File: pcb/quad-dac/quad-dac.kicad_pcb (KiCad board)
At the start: 2 copper layers, 90 x 90 mm, 18 parts, among them J1 Power+SPI, J2 CV_OUT, U1 AD5754R

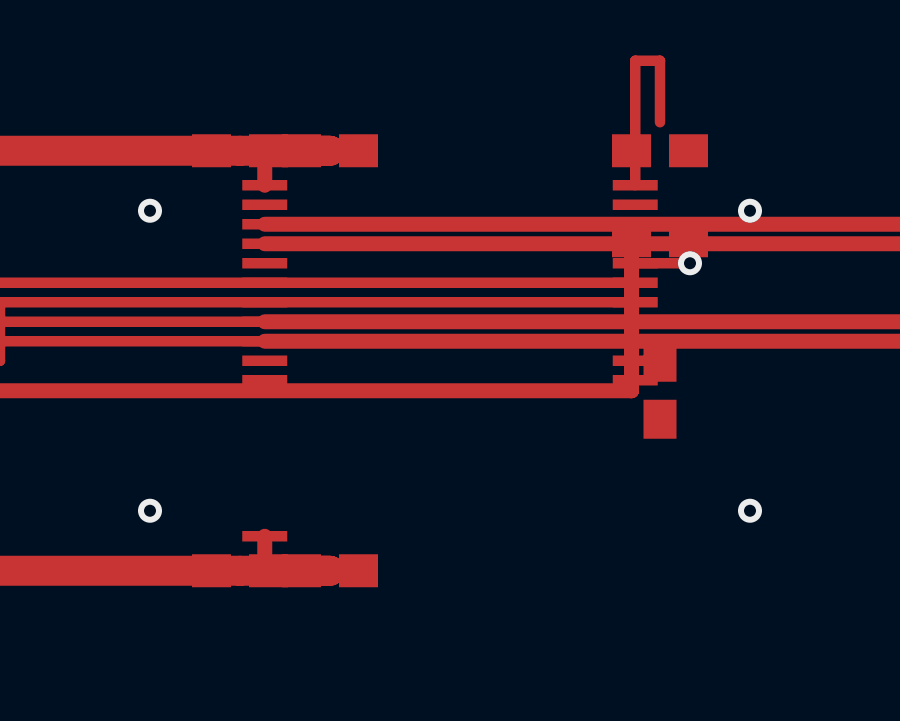
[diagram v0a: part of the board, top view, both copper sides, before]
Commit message: pcbs
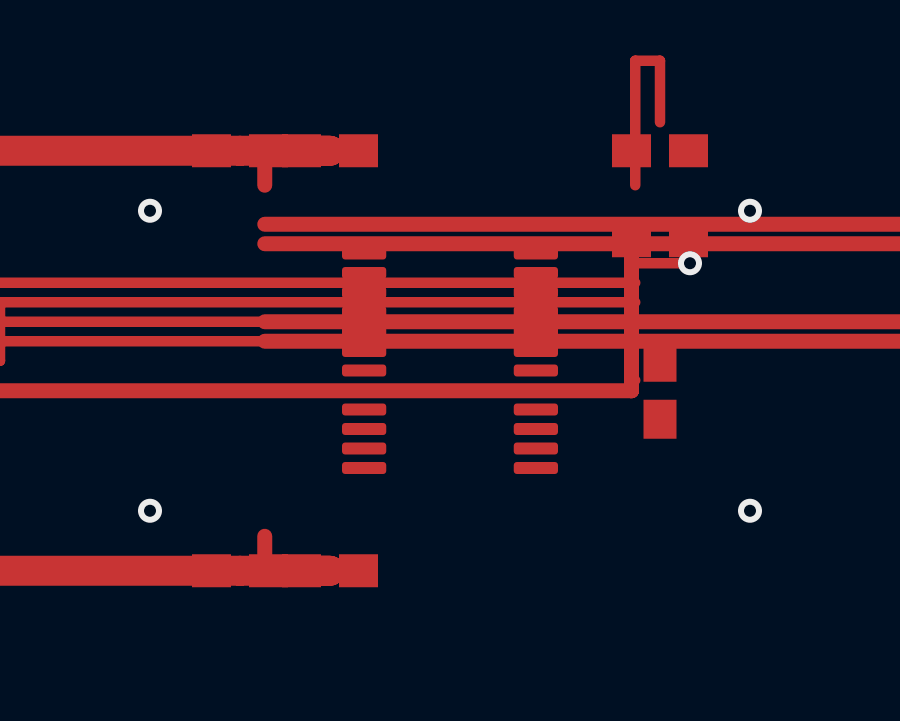
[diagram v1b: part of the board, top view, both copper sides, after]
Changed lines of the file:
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@@
   ;; =========================================================================
   ;; ── U1: AD5754R — TSSOP-24 ────────────────────────────────────────────
+  ;; Pin mapping: AD5754R pin 1 (AVSS) at top-left → KiCad pad 1 at (-2.8625, 3.575)
+  ;; Counter-clockwise: pads 1-12 left side (top→bottom), pads 13-24 right side (bottom→top)
   (footprint "Package_SO:TSSOP-24_4.4x7.8mm_P0.65mm"
     (layer "F.Cu")
@@
     (property "Value" "AD5754R" (at 45 52 0) (layer "F.Fab")
       (effects (font (size 1.0 1.0) (thickness 0.15))))
-    (pad "1" smd rect (at -6.175 -5.85 0) (size 1.5 0.35) (layers "F.Cu" "F.Paste" "F.Mask") (net 2))
-    (pad "2" smd rect (at -6.175 -5.2 0) (size 1.5 0.35) (layers "F.Cu" "F.Paste" "F.Mask") (net 4))
-    (pad "3" smd rect (at -6.175 -4.55 0) (size 1.5 0.35) (layers "F.Cu" "F.Paste" "F.Mask") (net 9))
-    (pad "4" smd rect (at -6.175 -3.9 0) (size 1.5 0.35) (layers "F.Cu" "F.Paste" "F.Mask") (net 10))
-    (pad "5" smd rect (at -6.175 -3.25 0) (size 1.5 0.35) (layers "F.Cu" "F.Paste" "F.Mask") (net 0))
-    (pad "6" smd rect (at -6.175 -2.6 0) (size 1.5 0.35) (layers "F.Cu" "F.Paste" "F.Mask") (net 0))
-    (pad "7" smd rect (at -6.175 -1.95 0) (size 1.5 0.35) (layers "F.Cu" "F.Paste" "F.Mask") (net 0))
-    (pad "8" smd rect (at -6.175 -1.3 0) (size 1.5 0.35) (layers "F.Cu" "F.Paste" "F.Mask") (net 11))
-    (pad "9" smd rect (at -6.175 -0.65 0) (size 1.5 0.35) (layers "F.Cu" "F.Paste" "F.Mask") (net 12))
-    (pad "10" smd rect (at -6.175 0.0 0) (size 1.5 0.35) (layers "F.Cu" "F.Paste" "F.Mask") (net 4))
-    (pad "11" smd rect (at -6.175 0.65 0) (size 1.5 0.35) (layers "F.Cu" "F.Paste" "F.Mask") (net 4))
-    (pad "12" smd rect (at 6.175 0.65 0) (size 1.5 0.35) (layers "F.Cu" "F.Paste" "F.Mask") (net 3))
-    (pad "13" smd rect (at 6.175 0.0 0) (size 1.5 0.35) (layers "F.Cu" "F.Paste" "F.Mask") (net 4))
-    (pad "14" smd rect (at 6.175 -0.65 0) (size 1.5 0.35) (layers "F.Cu" "F.Paste" "F.Mask") (net 6))
-    (pad "15" smd rect (at 6.175 -1.3 0) (size 1.5 0.35) (layers "F.Cu" "F.Paste" "F.Mask") (net 7))
-    (pad "16" smd rect (at 6.175 -1.95 0) (size 1.5 0.35) (layers "F.Cu" "F.Paste" "F.Mask") (net 5))
-    (pad "17" smd rect (at 6.175 -2.6 0) (size 1.5 0.35) (layers "F.Cu" "F.Paste" "F.Mask") (net 8))
-    (pad "18" smd rect (at 6.175 -3.25 0) (size 1.5 0.35) (layers "F.Cu" "F.Paste" "F.Mask") (net 4))
-    (pad "19" smd rect (at 6.175 -3.9 0) (size 1.5 0.35) (layers "F.Cu" "F.Paste" "F.Mask") (net 14))
-    (pad "20" smd rect (at 6.175 -4.55 0) (size 1.5 0.35) (layers "F.Cu" "F.Paste" "F.Mask") (net 0))
-    (pad "21" smd rect (at 6.175 -5.2 0) (size 1.5 0.35) (layers "F.Cu" "F.Paste" "F.Mask") (net 4))
-    (pad "22" smd rect (at 6.175 -5.85 0) (size 1.5 0.35) (layers "F.Cu" "F.Paste" "F.Mask") (net 13))
-    (pad "23" smd rect (at -6.175 0.65 0) (size 1.5 0.35) (layers "F.Cu" "F.Paste" "F.Mask") (net 4))
-    (pad "24" smd rect (at -6.175 5.85 0) (size 1.5 0.35) (layers "F.Cu" "F.Paste" "F.Mask") (net 1))
+    (pad "1" smd roundrect (at -2.8625 3.575) (size 1.475 0.4) (layers "F.Cu" "F.Paste" "F.Mask") (net 2) (roundrect_rratio 0.25))
+    (pad "2" smd roundrect (at -2.8625 2.925) (size 1.475 0.4) (layers "F.Cu" "F.Paste" "F.Mask") (net 4) (roundrect_rratio 0.25))
+    (pad "3" smd roundrect (at -2.8625 2.275) (size 1.475 0.4) (layers "F.Cu" "F.Paste" "F.Mask") (net 9) (roundrect_rratio 0.25))
+    (pad "4" smd roundrect (at -2.8625 1.625) (size 1.475 0.4) (layers "F.Cu" "F.Paste" "F.Mask") (net 10) (roundrect_rratio 0.25))
+    (pad "5" smd roundrect (at -2.8625 0.975) (size 1.475 0.4) (layers "F.Cu" "F.Paste" "F.Mask") (net 0) (roundrect_rratio 0.25))
+    (pad "6" smd roundrect (at -2.8625 0.325) (size 1.475 0.4) (layers "F.Cu" "F.Paste" "F.Mask") (net 0) (roundrect_rratio 0.25))
+    (pad "7" smd roundrect (at -2.8625 -0.325) (size 1.475 0.4) (layers "F.Cu" "F.Paste" "F.Mask") (net 0) (roundrect_rratio 0.25))
+    (pad "8" smd roundrect (at -2.8625 -0.975) (size 1.475 0.4) (layers "F.Cu" "F.Paste" "F.Mask") (net 11) (roundrect_rratio 0.25))
+    (pad "9" smd roundrect (at -2.8625 -1.625) (size 1.475 0.4) (layers "F.Cu" "F.Paste" "F.Mask") (net 12) (roundrect_rratio 0.25))
+    (pad "10" smd roundrect (at -2.8625 -2.275) (size 1.475 0.4) (layers "F.Cu" "F.Paste" "F.Mask") (net 4) (roundrect_rratio 0.25))
+    (pad "11" smd roundrect (at -2.8625 -2.925) (size 1.475 0.4) (layers "F.Cu" "F.Paste" "F.Mask") (net 4) (roundrect_rratio 0.25))
+    (pad "12" smd roundrect (at -2.8625 -3.575) (size 1.475 0.4) (layers "F.Cu" "F.Paste" "F.Mask") (net 3) (roundrect_rratio 0.25))
+    (pad "13" smd roundrect (at 2.8625 -3.575) (size 1.475 0.4) (layers "F.Cu" "F.Paste" "F.Mask") (net 4) (roundrect_rratio 0.25))
+    (pad "14" smd roundrect (at 2.8625 -2.925) (size 1.475 0.4) (layers "F.Cu" "F.Paste" "F.Mask") (net 6) (roundrect_rratio 0.25))
+    (pad "15" smd roundrect (at 2.8625 -2.275) (size 1.475 0.4) (layers "F.Cu" "F.Paste" "F.Mask") (net 7) (roundrect_rratio 0.25))
+    (pad "16" smd roundrect (at 2.8625 -1.625) (size 1.475 0.4) (layers "F.Cu" "F.Paste" "F.Mask") (net 5) (roundrect_rratio 0.25))
+    (pad "17" smd roundrect (at 2.8625 -0.975) (size 1.475 0.4) (layers "F.Cu" "F.Paste" "F.Mask") (net 8) (roundrect_rratio 0.25))
+    (pad "18" smd roundrect (at 2.8625 -0.325) (size 1.475 0.4) (layers "F.Cu" "F.Paste" "F.Mask") (net 4) (roundrect_rratio 0.25))
+    (pad "19" smd roundrect (at 2.8625 0.325) (size 1.475 0.4) (layers "F.Cu" "F.Paste" "F.Mask") (net 14) (roundrect_rratio 0.25))
+    (pad "20" smd roundrect (at 2.8625 0.975) (size 1.475 0.4) (layers "F.Cu" "F.Paste" "F.Mask") (net 0) (roundrect_rratio 0.25))
+    (pad "21" smd roundrect (at 2.8625 1.625) (size 1.475 0.4) (layers "F.Cu" "F.Paste" "F.Mask") (net 4) (roundrect_rratio 0.25))
+    (pad "22" smd roundrect (at 2.8625 2.275) (size 1.475 0.4) (layers "F.Cu" "F.Paste" "F.Mask") (net 13) (roundrect_rratio 0.25))
+    (pad "23" smd roundrect (at 2.8625 2.925) (size 1.475 0.4) (layers "F.Cu" "F.Paste" "F.Mask") (net 4) (roundrect_rratio 0.25))
+    (pad "24" smd roundrect (at 2.8625 3.575) (size 1.475 0.4) (layers "F.Cu" "F.Paste" "F.Mask") (net 1) (roundrect_rratio 0.25))
   )
   ;; ── J1: 2x5 Power+SPI Header ──────────────────────────────────────────
